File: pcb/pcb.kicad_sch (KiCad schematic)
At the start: 43 parts, among them J1 Conn_01x02_Socket, J2 Conn_01x04_Socket, U1 AP2112K-3.3TRG1, U2 W25Q16JVUXIQ, U3 RP2040, U4 DS4432U+T&amp;R, U5 AD8403ARUZ1-REEL, U6 ADG801BRTZ-REEL7, Y2 Crystal_GND24_Small

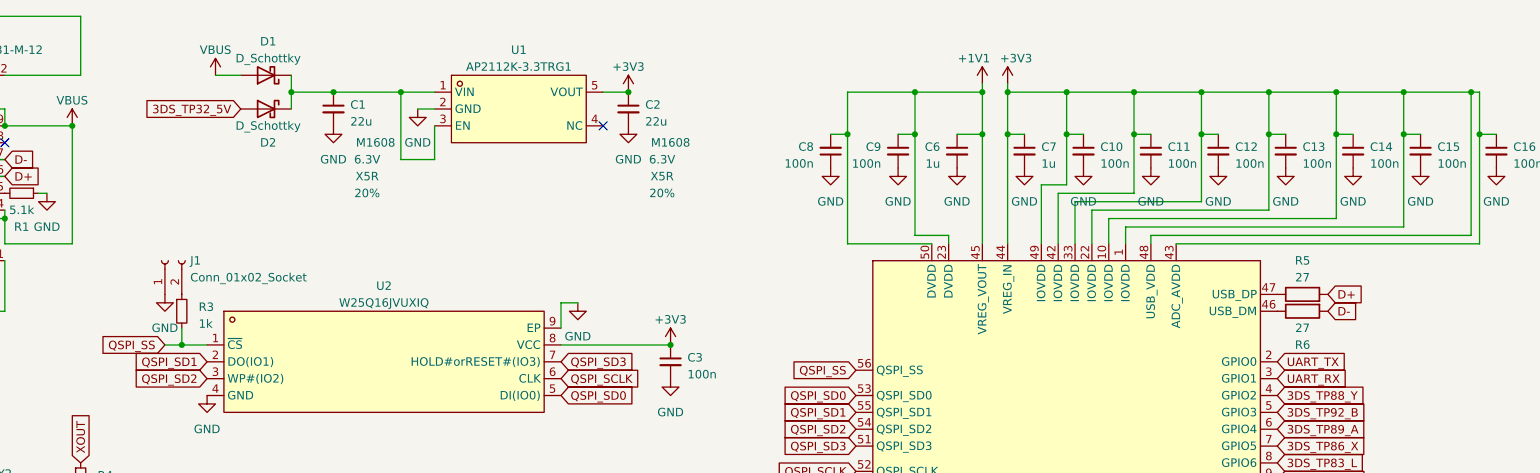
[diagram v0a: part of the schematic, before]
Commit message: flex
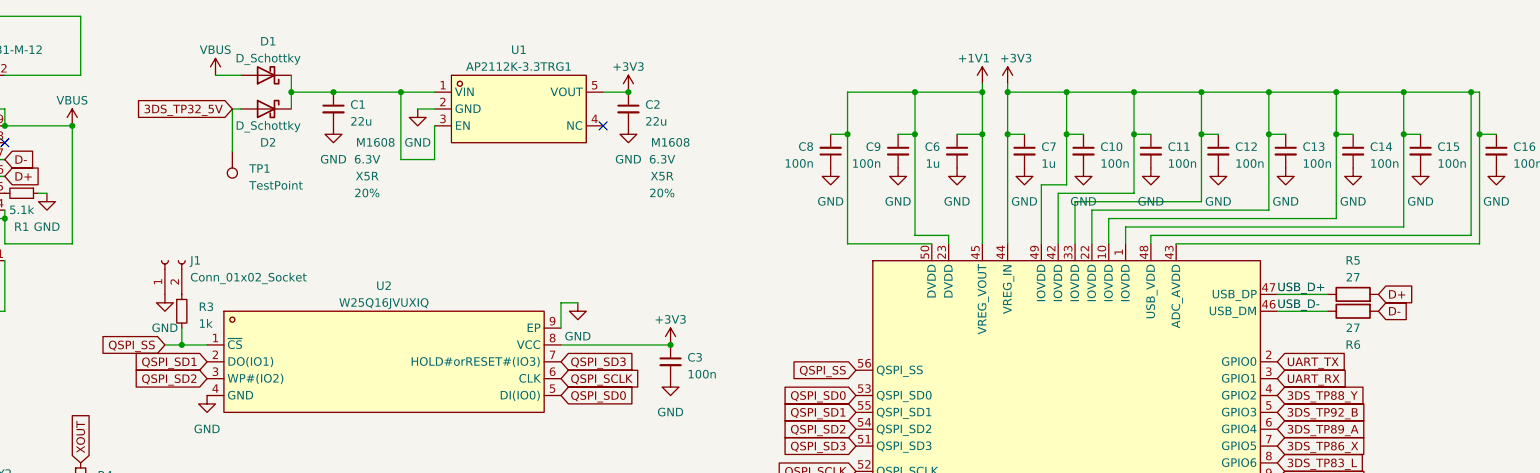
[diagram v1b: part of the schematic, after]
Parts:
- added TP1: TestPoint, TestPoint:TestPoint_Pad_D1.5mm, symbol Connector:TestPoint
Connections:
- net 3DS_TP32_5V: now also TP1.1
- net USB_D-: now reaches R6.1, U3.46 (USB_DM)
- net USB_D+: now reaches R5.1, U3.47 (USB_DP)
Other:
- moved on the sheet: R5, R6
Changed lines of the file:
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@@
+    (stroke (width 0) (type default))
+  )
+  (wire (pts (xy 245.11 55.88) (xy 237.49 55.88))
     (stroke (width 0) (type default))
   )
@@
     (stroke (width 0) (type default))
   )
+  (wire (pts (xy 237.49 58.42) (xy 245.11 58.42))
+    (stroke (width 0) (type default))
+  )
   (wire (pts (xy 45.72 44.45) (xy 45.72 43.18))
     (stroke (width 0) (type default))
@@
     (stroke (width 0) (type default))
   )
+  (wire (pts (xy 80.01 27.94) (xy 81.28 27.94))
+    (stroke (width 0) (type default))
+  )
   (wire (pts (xy 182.88 25.4) (xy 182.88 31.75))
     (stroke (width 0) (type default))
@@
     (stroke (width 0) (type default))
   )
+  (wire (pts (xy 80.01 34.29) (xy 80.01 27.94))
+    (stroke (width 0) (type default))
+  )
   (wire (pts (xy 33.02 58.42) (xy 35.56 58.42))
     (stroke (width 0) (type default))
@@
   )
   (text "Not assigned to CS, a normal GPIO." (at 247.65 116.84 0)
+    (effects (font (size 1.27 1.27)) (justify left bottom))
+  )
+  (label "USB_D-" (at 237.49 58.42 0) (fields_autoplaced)
+    (effects (font (size 1.27 1.27)) (justify left bottom))
+  )
+  (label "USB_D+" (at 237.49 55.88 0) (fields_autoplaced)
     (effects (font (size 1.27 1.27)) (justify left bottom))
   )
@@
     )
   )
-  (global_label "3DS_TP32_5V" (shape input) (at 81.28 27.94 180) (fields_autoplaced)
+  (global_label "3DS_TP32_5V" (shape input) (at 80.01 27.94 180) (fields_autoplaced)
     (effects (font (size 1.27 1.27)) (justify right))
-    (property "Intersheetrefs" "${INTERSHEET_REFS}" (at 65.7953 27.94 0)
+    (property "Intersheetrefs" "${INTERSHEET_REFS}" (at 64.5253 27.94 0)
       (effects (font (size 1.27 1.27)) (justify right) hide)
     )
@@
     )
   )
-  (global_label "D-" (shape input) (at 245.11 58.42 0) (fields_autoplaced)
-    (effects (font (size 1.27 1.27)) (justify left))
-    (property "Intersheetrefs" "${INTERSHEET_REFS}" (at 250.8582 58.42 0)
+  (global_label "D-" (shape input) (at 252.73 58.42 0) (fields_autoplaced)
+    (effects (font (size 1.27 1.27)) (justify left))
+    (property "Intersheetrefs" "${INTERSHEET_REFS}" (at 258.4782 58.42 0)
       (effects (font (size 1.27 1.27)) (justify left) hide)
     )
@@
     )
   )
-  (global_label "D+" (shape input) (at 245.11 55.88 0) (fields_autoplaced)
-    (effects (font (size 1.27 1.27)) (justify left))
-    (property "Intersheetrefs" "${INTERSHEET_REFS}" (at 250.8582 55.88 0)
+  (global_label "D+" (shape input) (at 252.73 55.88 0) (fields_autoplaced)
+    (effects (font (size 1.27 1.27)) (justify left))
+    (property "Intersheetrefs" "${INTERSHEET_REFS}" (at 258.4782 55.88 0)
       (effects (font (size 1.27 1.27)) (justify left) hide)
     )
@@
     )
   )
-  (symbol (lib_id "Device:R") (at 241.3 55.88 90) (unit 1)
-    (in_bom yes) (on_board yes) (dnp no) (fields_autoplaced)
-    (property "Reference" "R5" (at 241.3 50.8 90)
-      (effects (font (size 1.27 1.27)))
-    )
-    (property "Value" "27" (at 241.3 53.34 90)
-      (effects (font (size 1.27 1.27)))
-    )
-    (property "Footprint" "Resistor_SMD:R_0402_1005Metric" (at 241.3 57.658 90)
-      (effects (font (size 1.27 1.27)) hide)
-    )
-    (property "Datasheet" "~" (at 241.3 55.88 0)
-      (effects (font (size 1.27 1.27)) hide)
-    )
-    (property "LCSC" "C102938" (at 241.3 55.88 90)
+  (symbol (lib_id "Device:R") (at 248.92 55.88 90) (unit 1)
+    (in_bom yes) (on_board yes) (dnp no) (fields_autoplaced)
+    (property "Reference" "R5" (at 248.92 50.8 90)
+      (effects (font (size 1.27 1.27)))
+    )
+    (property "Value" "27" (at 248.92 53.34 90)
+      (effects (font (size 1.27 1.27)))
+    )
+    (property "Footprint" "Resistor_SMD:R_0402_1005Metric" (at 248.92 57.658 90)
+      (effects (font (size 1.27 1.27)) hide)
+    )
+    (property "Datasheet" "~" (at 248.92 55.88 0)
+      (effects (font (size 1.27 1.27)) hide)
+    )
+    (property "LCSC" "C102938" (at 248.92 55.88 90)
       (effects (font (size 1.27 1.27)) hide)
     )
@@
         (path "/4db5c0ae-dab5-4243-9886-99aa858b7752"
           (reference "R11") (unit 1)
+        )
+      )
+    )
+  )
+  (symbol (lib_id "Connector:TestPoint") (at 80.01 34.29 180) (unit 1)
+    (in_bom yes) (on_board yes) (dnp no) (fields_autoplaced)
+    (property "Reference" "TP1" (at 82.55 36.957 0)
+      (effects (font (size 1.27 1.27)) (justify right))
+    )
+    (property "Value" "TestPoint" (at 82.55 39.497 0)
+      (effects (font (size 1.27 1.27)) (justify right))
+    )
+    (property "Footprint" "TestPoint:TestPoint_Pad_D1.5mm" (at 74.93 34.29 0)
+      (effects (font (size 1.27 1.27)) hide)
+    )
+    (property "Datasheet" "~" (at 74.93 34.29 0)
+      (effects (font (size 1.27 1.27)) hide)
+    )
+    (pin "1")
+    (instances
+      (project "pcb"
+        (path "/4db5c0ae-dab5-4243-9886-99aa858b7752"
+          (reference "TP1") (unit 1)
         )
       )
@@
     )
   )
-  (symbol (lib_id "Device:R") (at 241.3 58.42 90) (mirror x) (unit 1)
+  (symbol (lib_id "Device:R") (at 248.92 58.42 90) (mirror x) (unit 1)
     (in_bom yes) (on_board yes) (dnp no)
-    (property "Reference" "R6" (at 241.3 63.5 90)
-      (effects (font (size 1.27 1.27)))
-    )
-    (property "Value" "27" (at 241.3 60.96 90)
-      (effects (font (size 1.27 1.27)))
-    )
-    (property "Footprint" "Resistor_SMD:R_0402_1005Metric" (at 241.3 56.642 90)
-      (effects (font (size 1.27 1.27)) hide)
-    )
-    (property "Datasheet" "~" (at 241.3 58.42 0)
-      (effects (font (size 1.27 1.27)) hide)
-    )
-    (property "LCSC" "C102938" (at 241.3 58.42 90)
-      (effects (font (size 1.27 1.27)) hide)
-    )
+    (property "Reference" "R6" (at 248.92 63.5 90)
+      (effects (font (size 1.27 1.27)))
+    )
+    (property "Value" "27" (at 248.92 60.96 90)
+      (effects (font (size 1.27 1.27)))
+    )
+    (property "Footprint" "Resistor_SMD:R_0402_1005Metric" (at 248.92 56.642 90)
+      (effects (font (size 1.27 1.27)) hide)
+    )
+    (property "Datasheet" "~" (at 248.92 58.42 0)
+      (effects (font (size 1.27 1.27)) hide)
+    )
+    (property "LCSC" "C102938" (at 248.92 58.42 90)
+      (effects (font (size 1.27 1.27)) hide)
+    )
